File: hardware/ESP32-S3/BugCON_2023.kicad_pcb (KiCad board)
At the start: 2 copper layers, 31 parts, among them J1 Conn_01x04_Pin, J2 Conn_01x04_Pin, J4 Battery, P1 USB_C_Plug_USB2.0, Q1 DMG3415U-7, SW1 RESET, SW2 GPIO, SW3 ON, U1 ESP32-S3-WROOM-1U-N16, U2 AP2112K-3.3

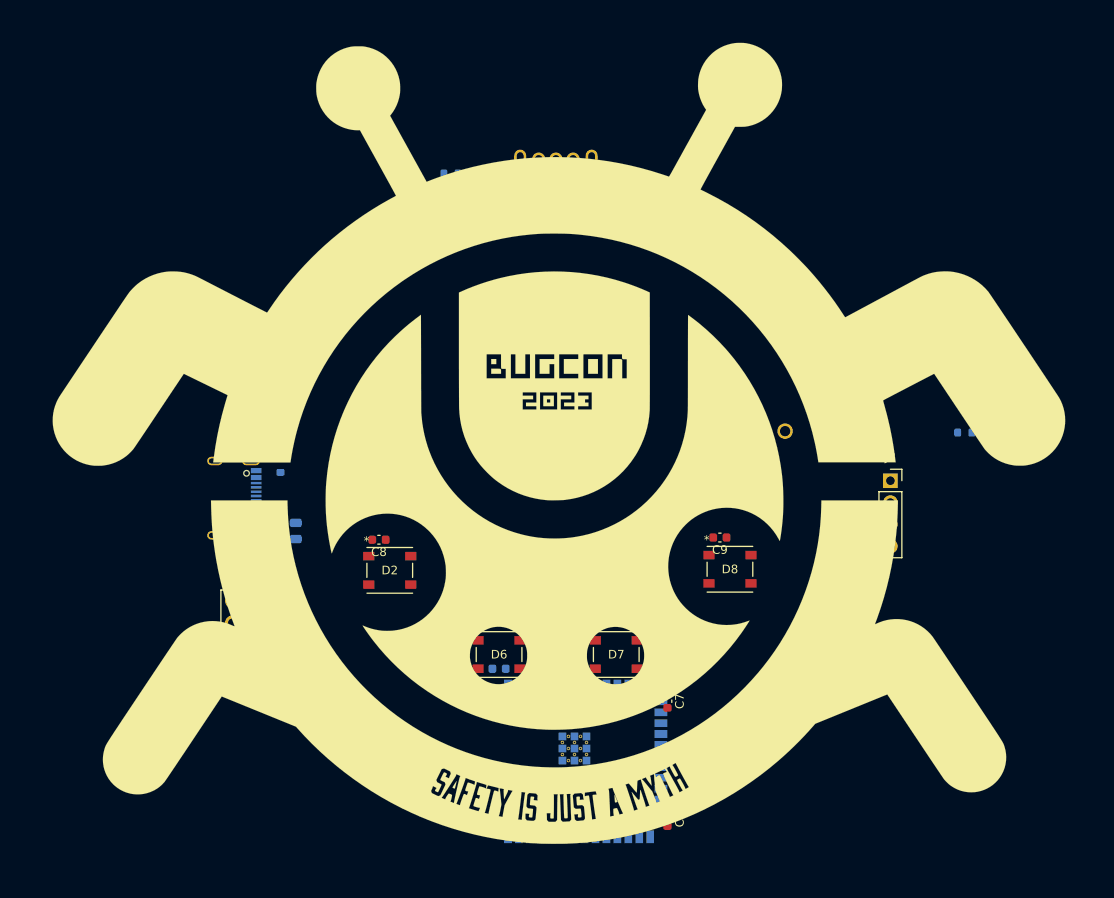
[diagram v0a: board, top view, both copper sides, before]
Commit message: First_route_Change_size
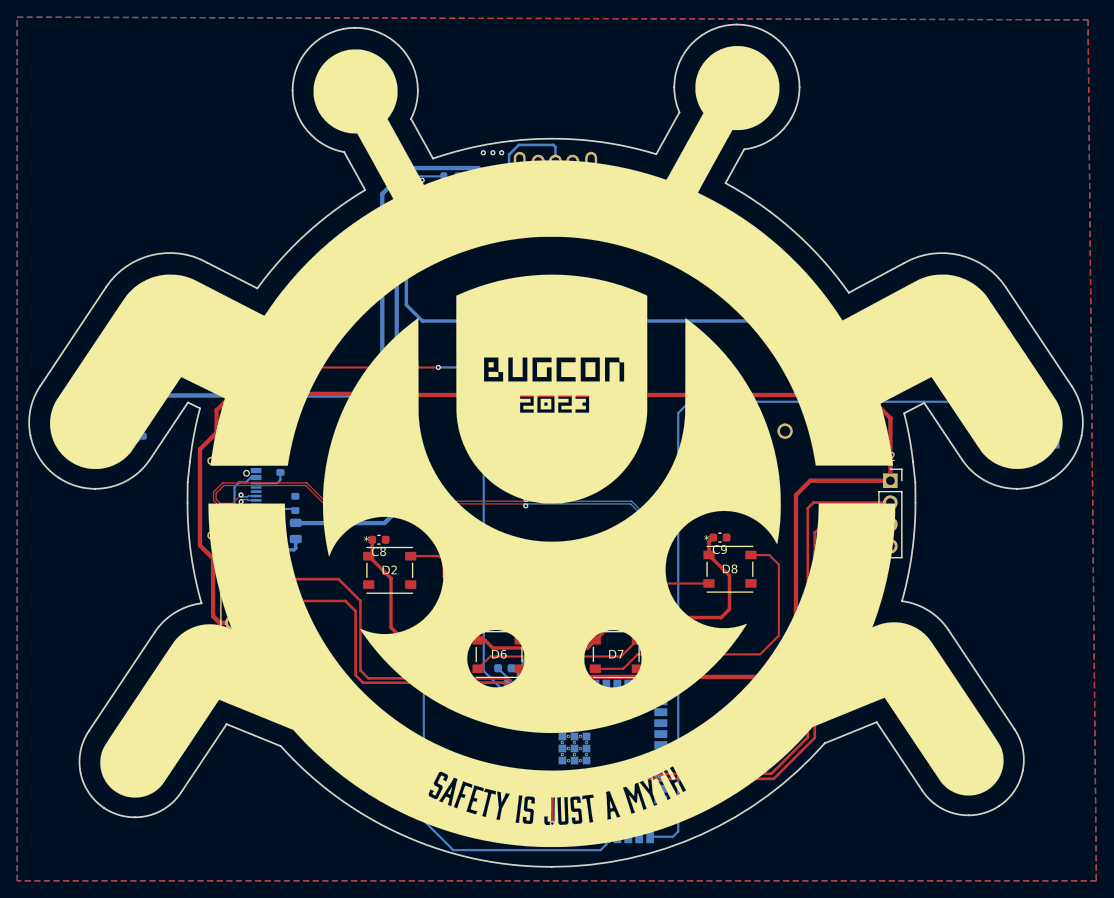
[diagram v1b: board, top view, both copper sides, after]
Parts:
- removed the Ref** at (143.1, 78.9)
- added Ref**: Val**, FootprintsB:Bugcon_svg, F.Cu at (144.1, 73.0)
- moved SW2 107.3 mm to (198.5, 70.8)
- moved SW1 106.5 mm to (90.8, 70.5)
- moved R1 95.5 mm to (96.0, 71.0), turned to 90 degrees
- moved C7 25.9 mm to (131.9, 96.2), turned to 90 degrees
- moved C6 22.8 mm to (155.6, 93.6), turned to 90 degrees
- moved R2 3.63 mm to (113.7, 79.6), turned to -90 degrees
- moved C2 0.66 mm to (138.1, 98.8)
- moved C3 0.60 mm to (141.1, 98.8)
- moved C1 0.56 mm to (144.1, 98.8)
- moved R4 0.33 mm to (131.8, 41.6)
- moved SW3 0.26 mm to (144.0, 39.8)
- turned F1 to 90 degrees
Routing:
- net +3V3: track 0.00 -> 256.3 mm, vias 0 -> 2
- net /RST: track 0.00 -> 106.0 mm, vias 0 -> 2
- net /BOOT: track 0.00 -> 98.2 mm
- net /D+: track 0.00 -> 79.0 mm, vias 0 -> 2
- net /D-: track 0.00 -> 77.7 mm, vias 0 -> 2
- net /TX: track 0.00 -> 76.3 mm, vias 0 -> 1
- net /RX: track 0.00 -> 71.9 mm, vias 0 -> 1
- net /PIN: track 0.00 -> 65.0 mm, vias 0 -> 1
- net +3.3V: track 0.00 -> 63.1 mm
- net /SDA: track 0.00 -> 60.4 mm, vias 0 -> 1
- net +BATT: track 0.00 -> 58.2 mm
- net VBUS: track 0.00 -> 57.5 mm
- net /SCL: track 0.00 -> 46.3 mm, vias 0 -> 1
- net Net-(D2-DIN): track 0.00 -> 37.0 mm
- net Net-(D7-DOUT): track 0.00 -> 34.9 mm
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- added copper zone on B.Cu, net GND
- added copper zone on F.Cu, net GND
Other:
- board outline added: 122.4 x 97.9 mm
